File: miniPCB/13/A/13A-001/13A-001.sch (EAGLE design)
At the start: 12 parts, among them U1 OPAMP_QUADTHD

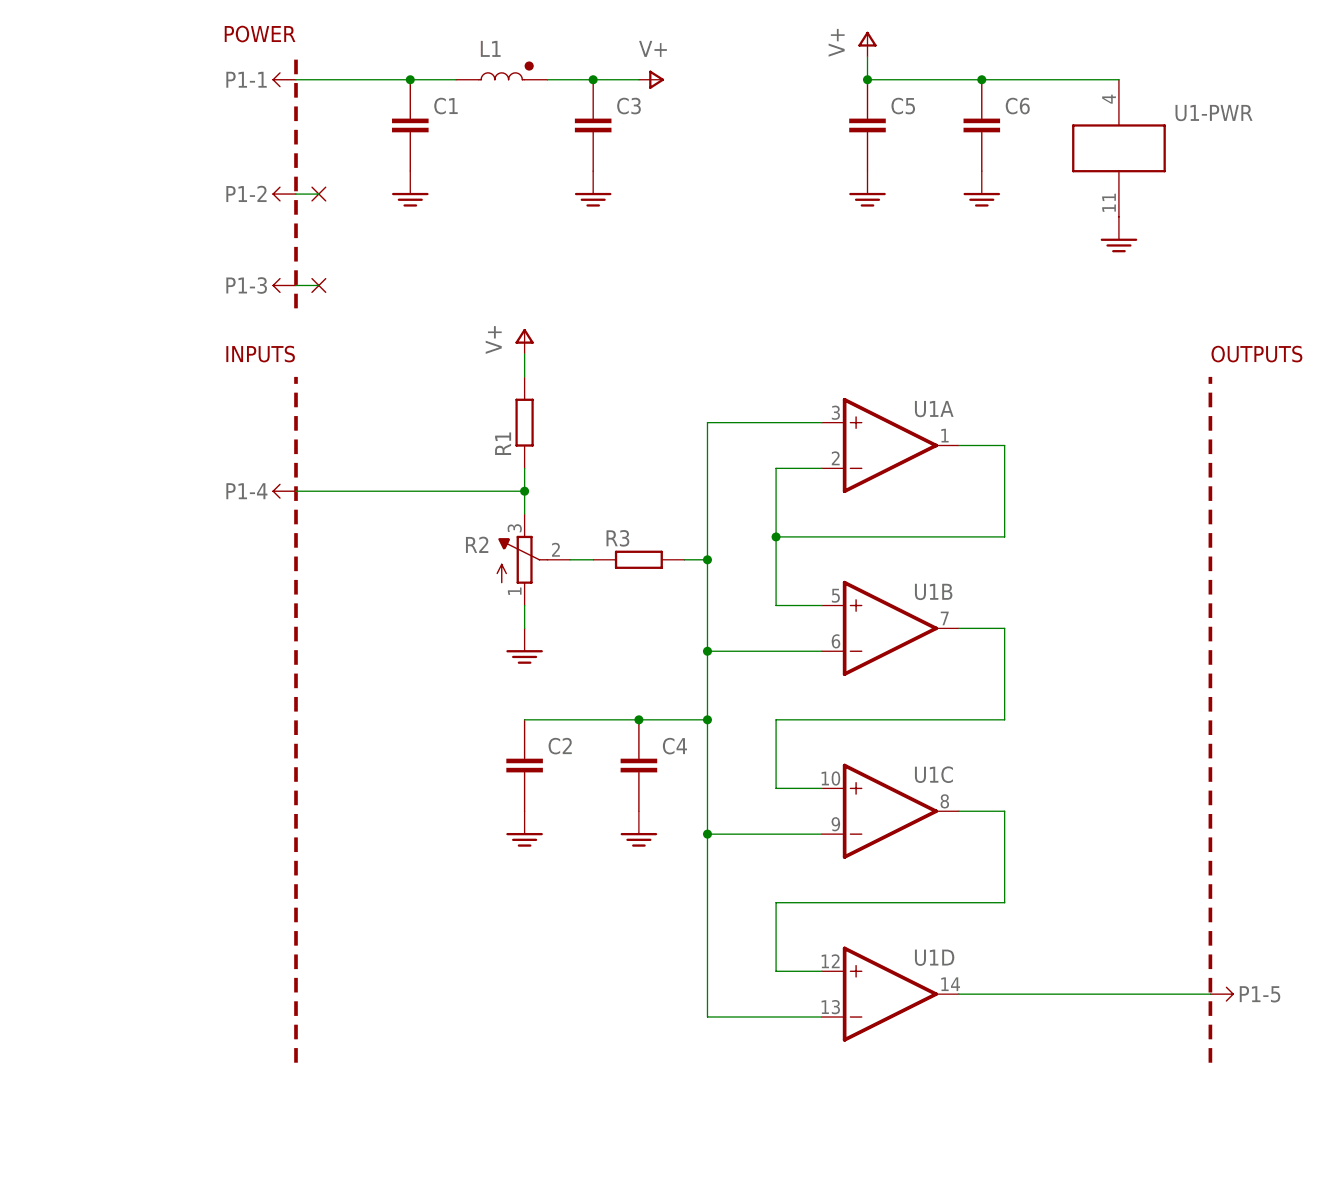
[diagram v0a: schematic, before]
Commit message: NM.03SEP2023
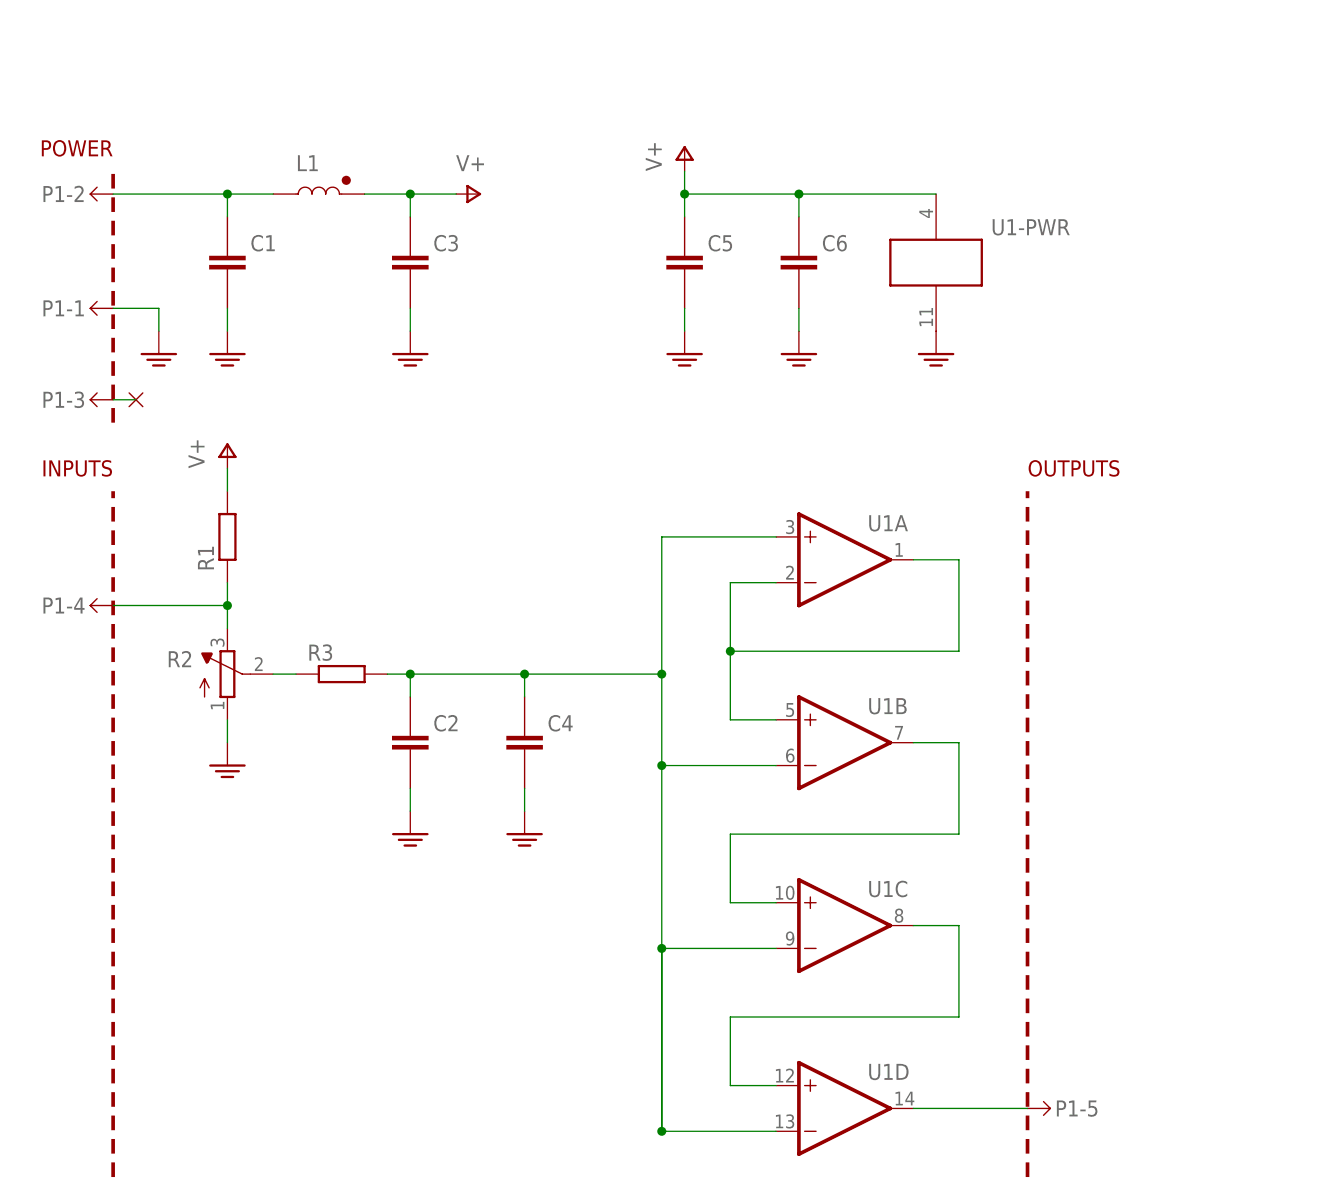
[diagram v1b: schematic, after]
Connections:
- removed net N$10: P1-2.1
- net GND: now also P1-1.1
- net N$5: now also P1-2.1; no longer P1-1.1
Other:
- moved on the sheet: C1, C2, C3, C4, C5, C6, L1, P1-1, P1-2, P1-3, P1-4, P1-5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
